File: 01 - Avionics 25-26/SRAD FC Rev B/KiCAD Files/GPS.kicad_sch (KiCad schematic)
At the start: 3 parts

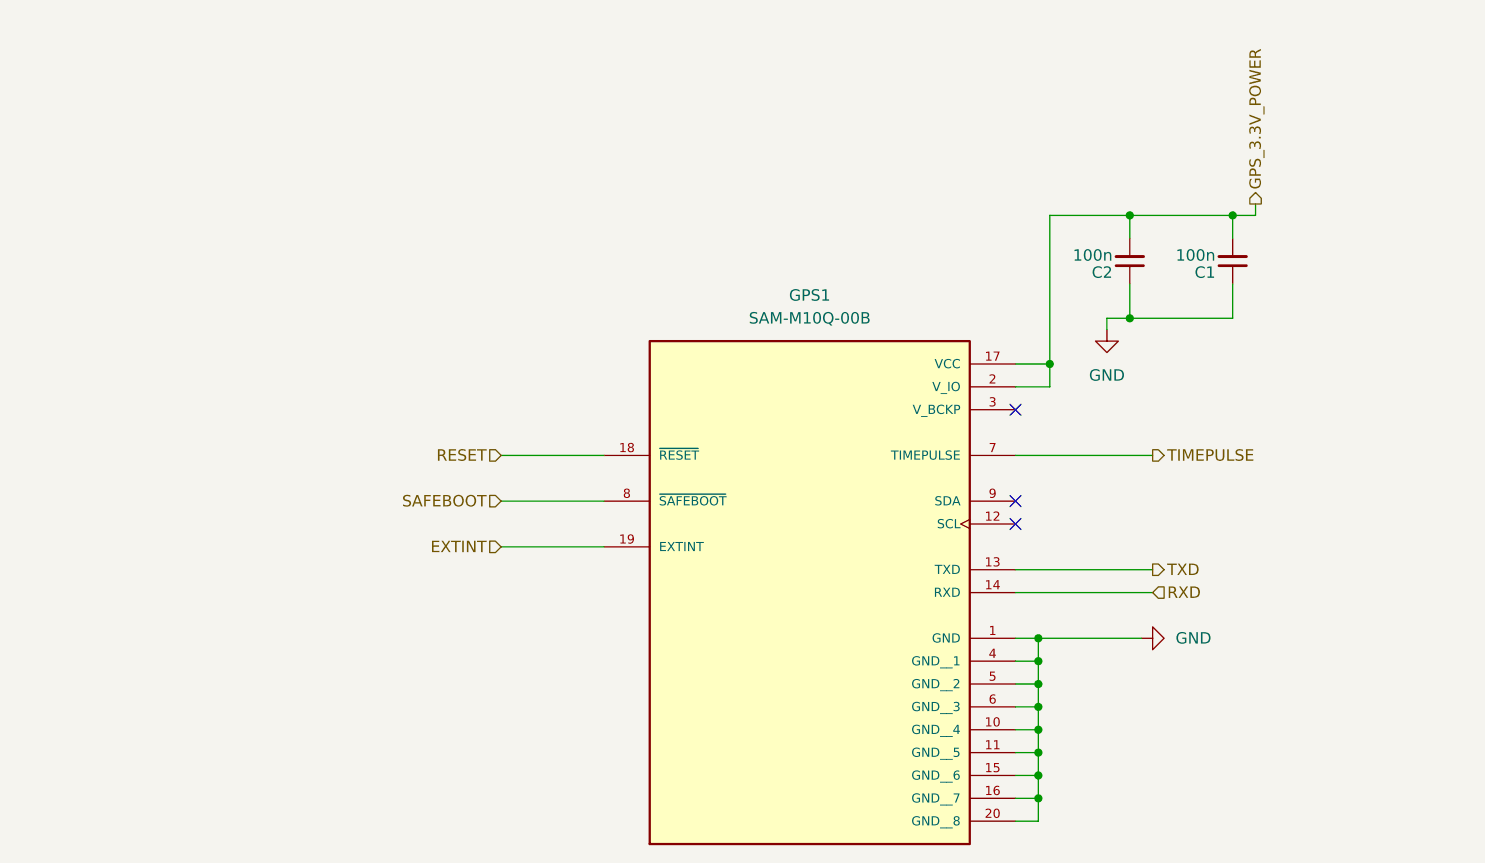
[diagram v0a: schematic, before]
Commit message: fixed some library symbold
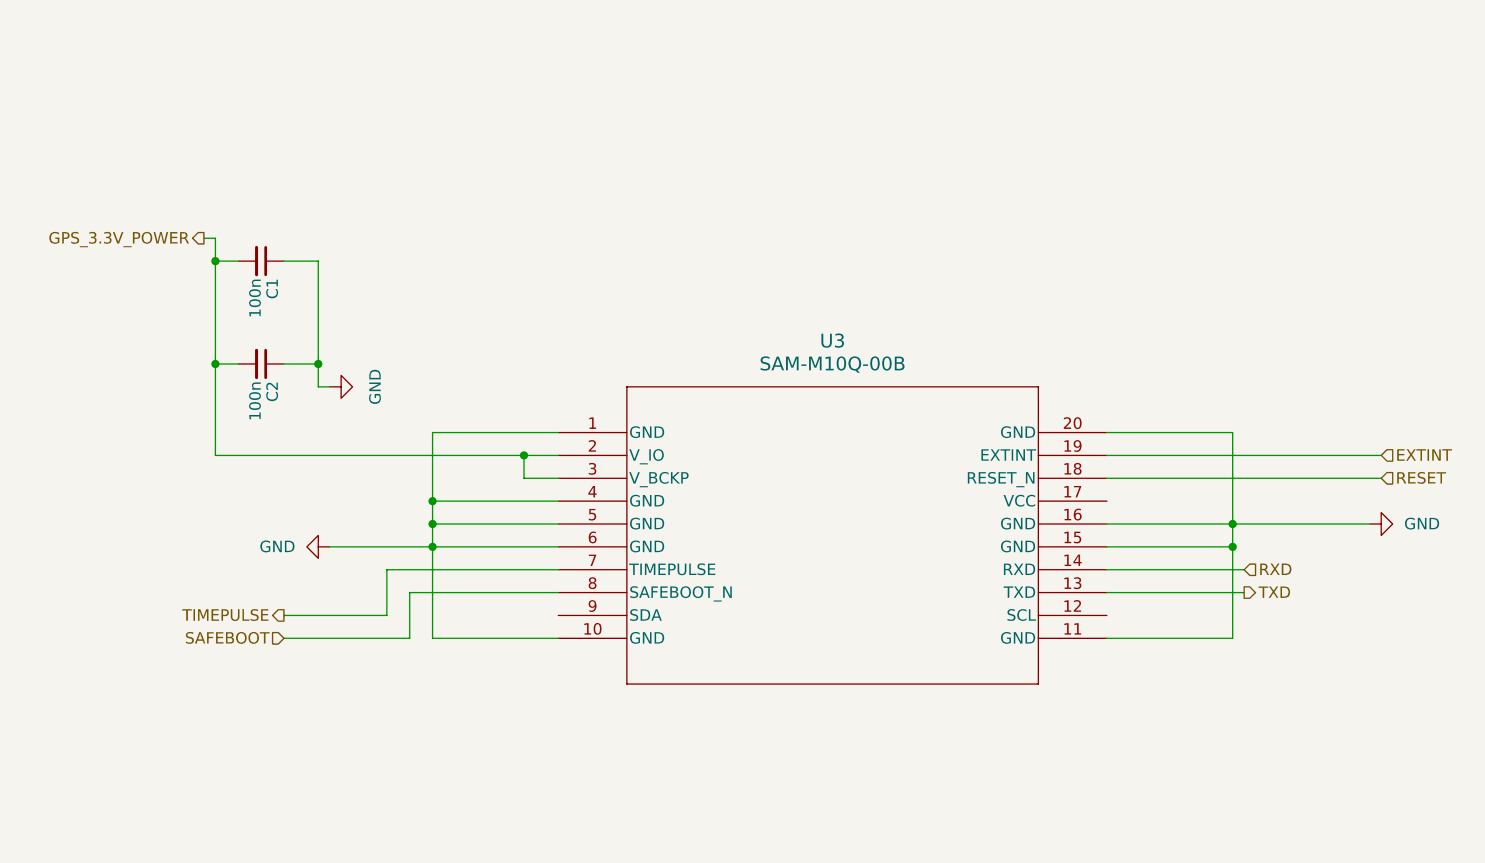
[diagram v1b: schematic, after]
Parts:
- removed GPS1: SAM-M10Q-00B, Package_LGA:ublox_LGA-53_4.5x4.5mm_Layout9x9_P0.5mm, symbol SAM-M10Q-00B:SAM-M10Q-00B
- added U3: SAM-M10Q-00B, SAM_M10Q_00B:SAM-M10Q_UBL, symbol SAM-M10Q-00B:SAM-M10Q-00B
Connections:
- net EXTINT: now also U3.19 (EXTINT)
- net GND: now also U3.1 (GND), U3.10 (GND), U3.11 (GND), U3.15 (GND), U3.16 (GND), U3.20 (GND), U3.4 (GND), U3.5 (GND), U3.6 (GND)
- net GPS_3.3V_POWER: now also U3.2 (V_IO), U3.3 (V_BCKP)
- net RESET: now also U3.18 (RESET_N)
- net RXD: now also U3.14 (RXD)
- net SAFEBOOT: now also U3.8 (SAFEBOOT_N)
- net TIMEPULSE: now also U3.7 (TIMEPULSE)
- net TXD: now also U3.13 (TXD)
- no-connect marks 3 -> 0
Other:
- moved on the sheet: C1, C2
